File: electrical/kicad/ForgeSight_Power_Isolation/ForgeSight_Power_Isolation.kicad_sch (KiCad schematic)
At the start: 33 parts, among them J1 24V/12V IN, J2 AUX_12V_OUT, J3 5V_ORANGE_PI_OUT, J4 TRIG_SENSOR_IN_24V, J5 ORANGE_PI_GPIO_HDR, U1 XL4015 (5V/4A Buck), U2 PC817, U3 PC817, U4 PC817, U5 PC817, U6 PC817

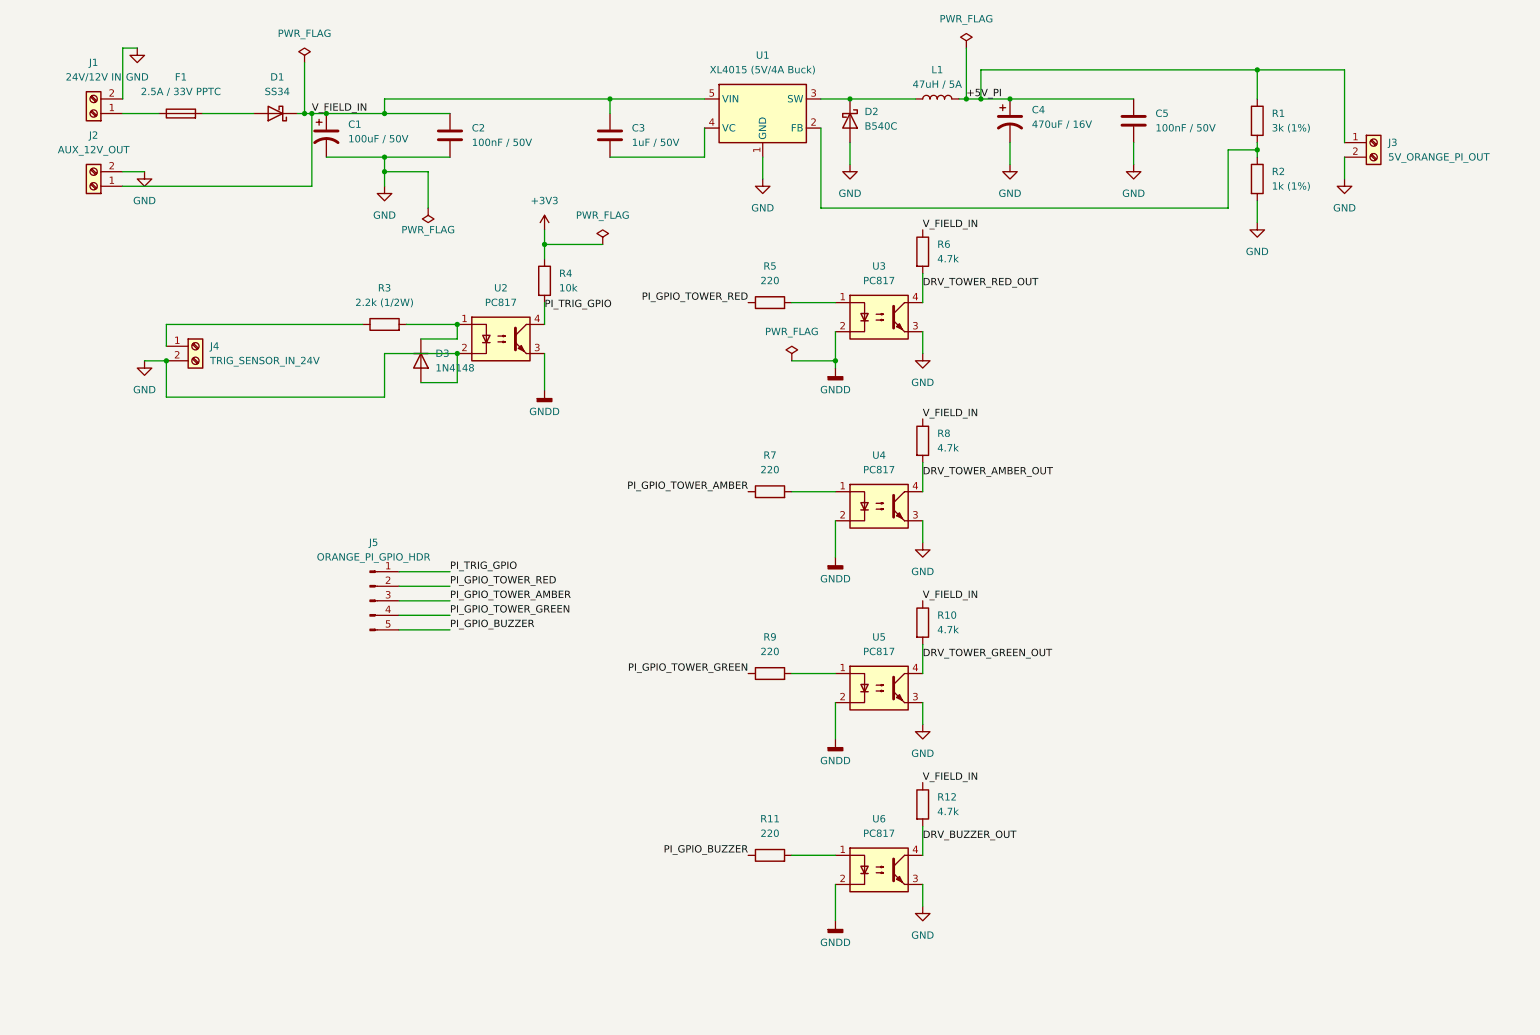
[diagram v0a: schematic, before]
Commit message: final electric schematics
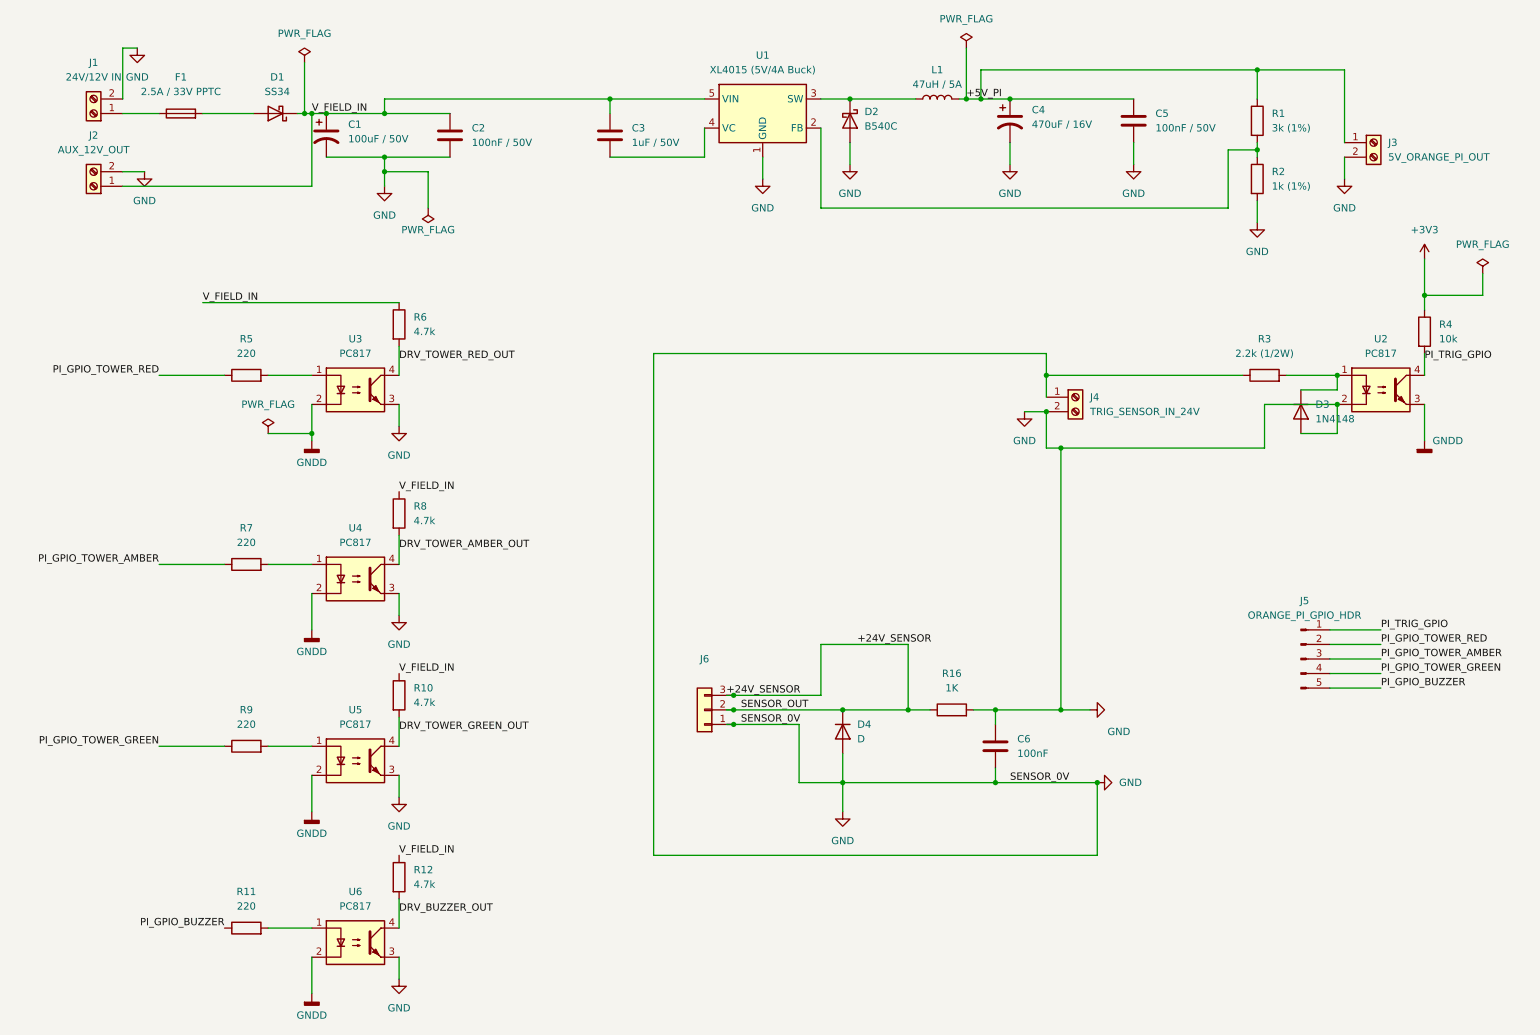
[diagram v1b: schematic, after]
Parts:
- added C6: 100nF, symbol Device:C
- added D4: D, Package_SON:WSON-8-1EP_6x5mm_P1.27mm_EP3.4x4mm, symbol Device:D
- added J6: Conn_01x03, Package_TO_SOT_SMD:TO-263-9_TabPin5, symbol Connector_Generic:Conn_01x03
- added R16: 1K, symbol Device:R
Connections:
- net GND: now also J4.1 (Pin_1), R3.1, C6.1, C6.2, D4.2 (A), J6.1 (Pin_1), R16.2
- new net +24V_SENSOR: D4.1 (K), J6.2 (Pin_2), J6.3 (Pin_3), R16.1
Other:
- moved on the sheet: D3, J4, J5, R10, R11, R12, R3, R4, R5, R6, R7, R8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
